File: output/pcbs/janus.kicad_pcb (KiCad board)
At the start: 2 copper layers, 180.2 x 117.5 mm, 55 parts

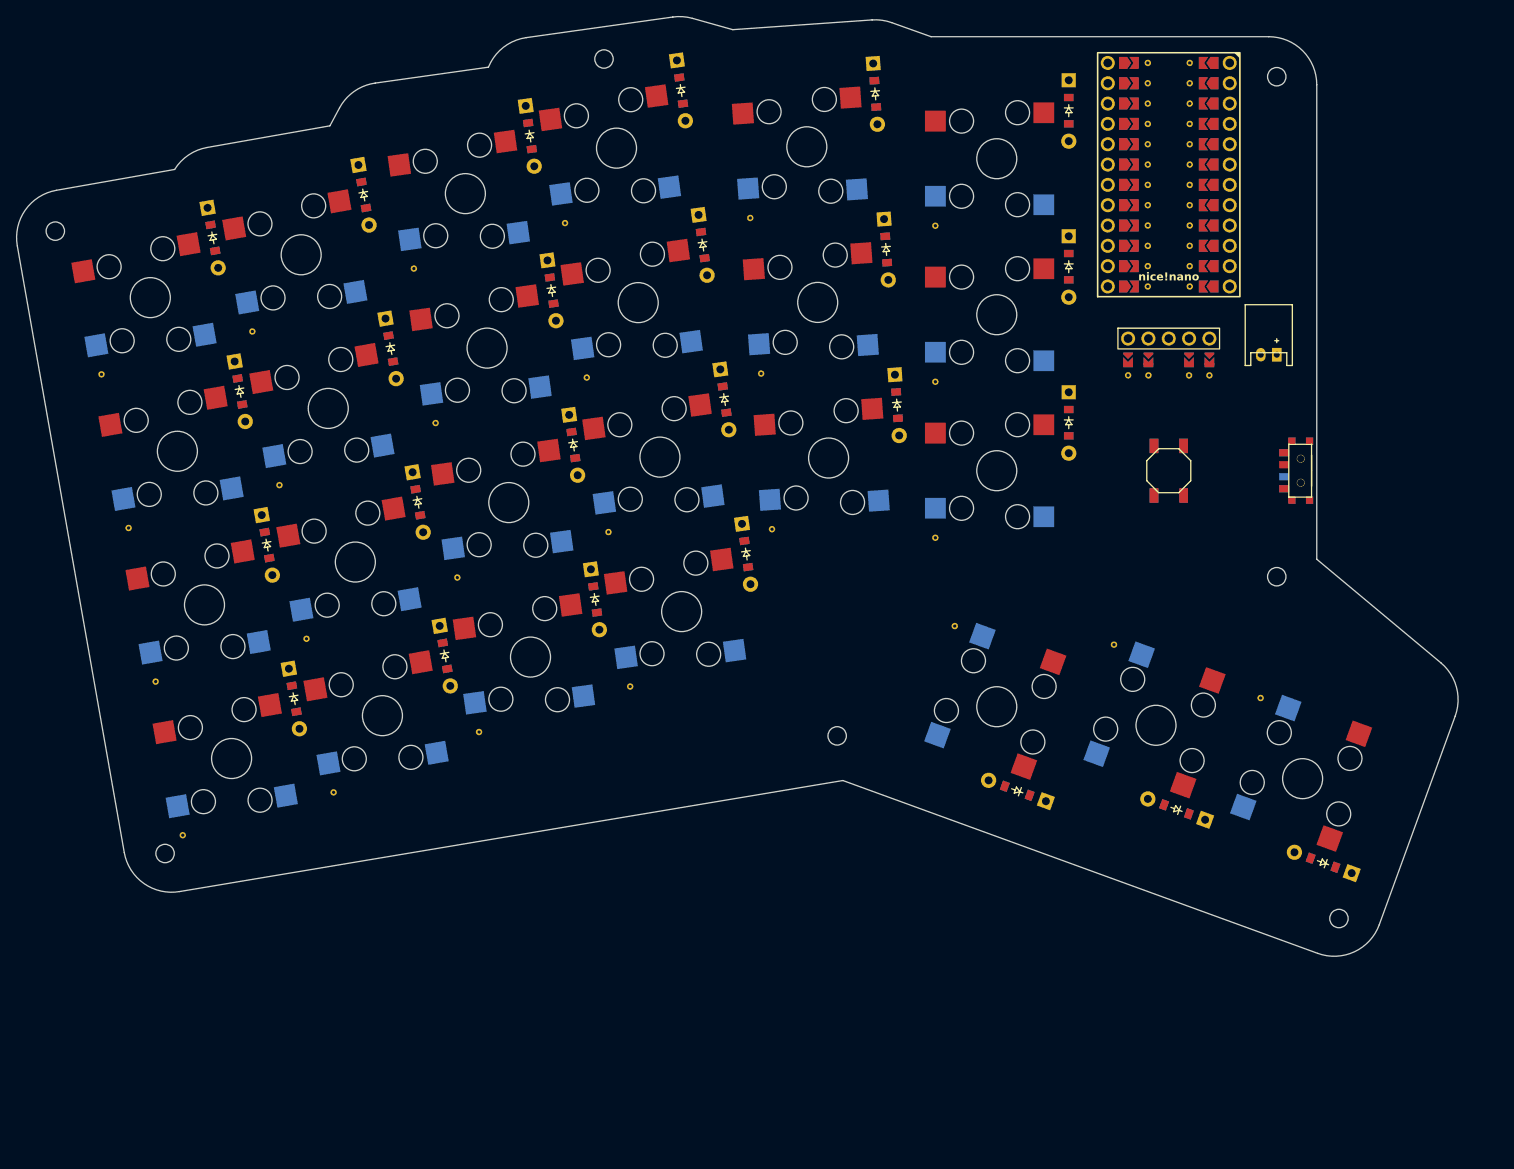
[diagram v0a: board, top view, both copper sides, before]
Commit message: generated output
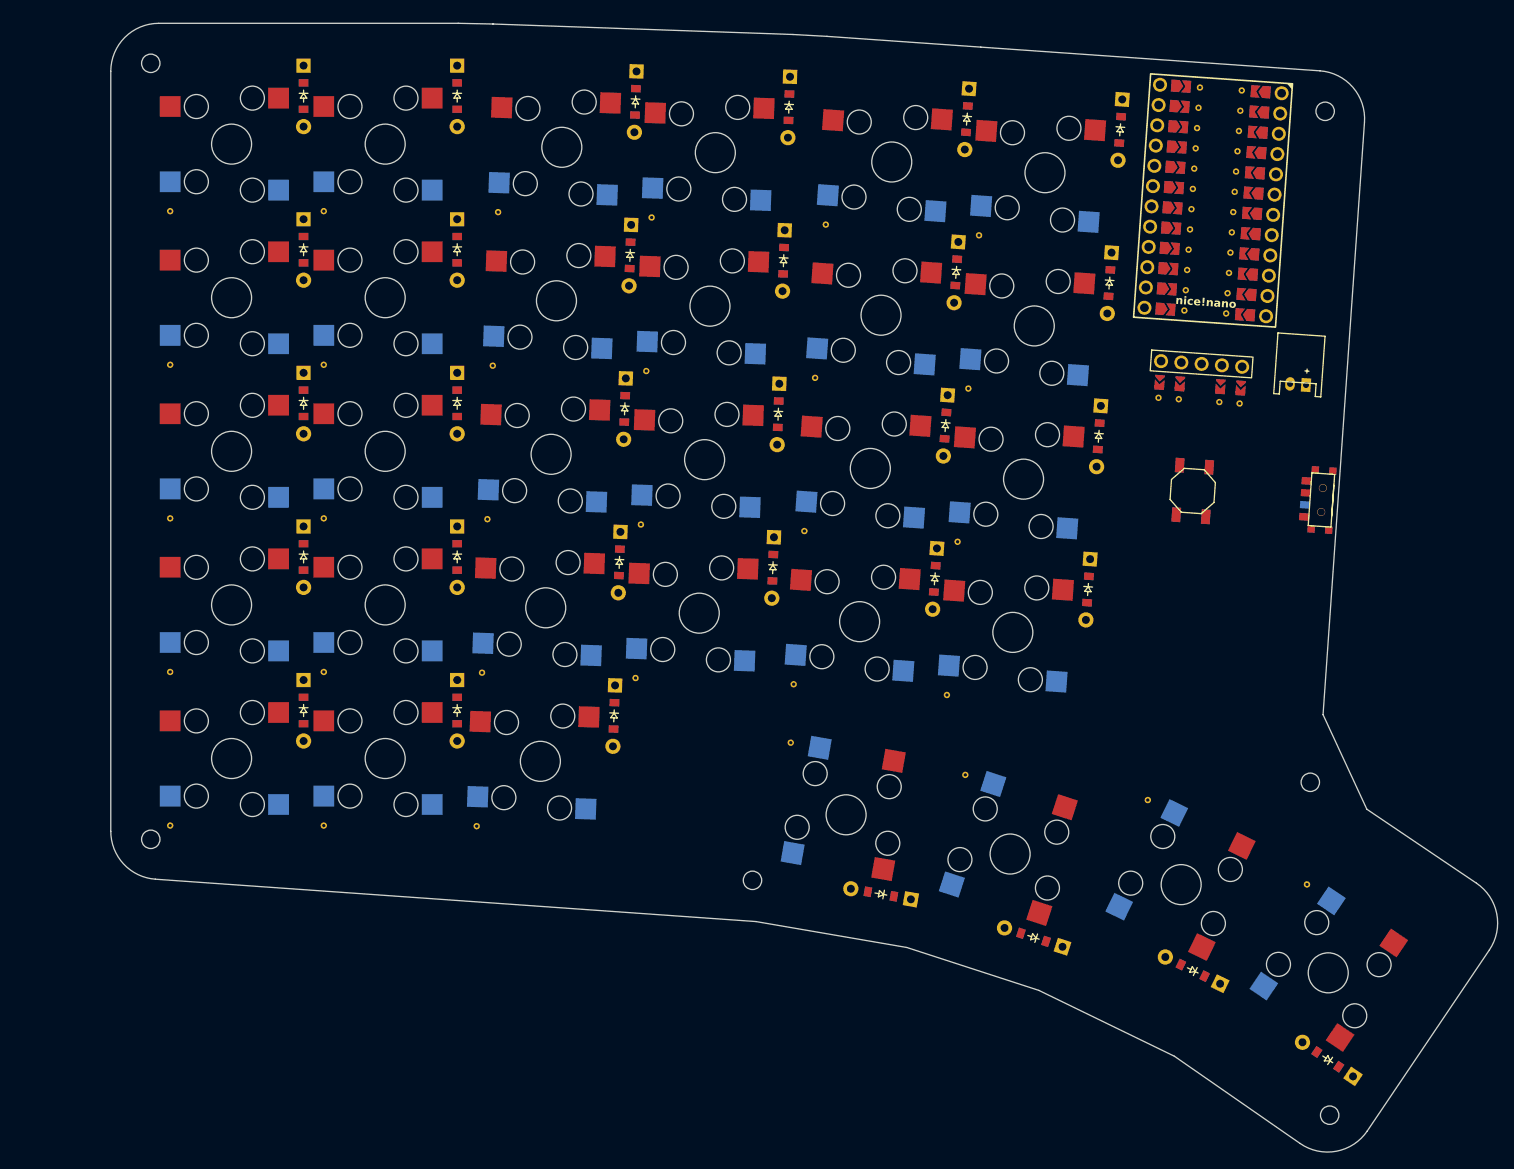
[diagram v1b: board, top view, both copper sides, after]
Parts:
- added D26: , ComboDiode, F.Cu at (159.7, 90.6)
- added D27: , ComboDiode, F.Cu at (161.1, 71.4)
- added D28: , ComboDiode, F.Cu at (131.2, 166.9)
- added D29: , ComboDiode, F.Cu at (150.2, 172.4)
- added D30: , ComboDiode, F.Cu at (170.1, 176.5)
- added D31: , ComboDiode, F.Cu at (187.0, 187.6)
- added S26: ks27, gateron-ks27, F.Cu at (150.3, 95.9)
- added S27: ks27, gateron-ks27, F.Cu at (151.7, 76.8)
- added S28: ks27, gateron-ks27, F.Cu at (126.8, 157.0)
- added S29: ks27, gateron-ks27, F.Cu at (147.3, 161.9)
- added S30: ks27, gateron-ks27, F.Cu at (168.7, 165.8)
- added S31: ks27, gateron-ks27, F.Cu at (187.1, 176.8)
- moved D23 84.2 mm to (141.9, 70.1), turned to -94 degrees
- moved S5 73.9 mm to (50.0, 73.2), turned to 0 degrees
- moved D5 72.2 mm to (59.0, 67.2), turned to -90 degrees
- moved S23 69.3 mm to (132.5, 75.4), turned to -4 degrees
- moved D16 60.7 mm to (117.7, 126.1), turned to -92 degrees
- moved D25 60.2 mm to (158.4, 109.7), turned to -94 degrees
- moved S16 59.0 mm to (108.5, 131.8), turned to -2 degrees
- moved D12 54.4 mm to (98.5, 125.5), turned to -92 degrees
- moved D11 53.7 mm to (97.8, 144.7), turned to -92 degrees
- moved S12 52.7 mm to (89.3, 131.2), turned to -2 degrees
- moved S11 52.1 mm to (88.6, 150.3), turned to -2 degrees
- moved S25 51.2 mm to (149.0, 115.1), turned to -4 degrees
- moved S9 48.5 mm to (69.2, 92.4), turned to 0 degrees
- moved S10 47.4 mm to (69.2, 73.2), turned to 0 degrees
- moved D9 47.0 mm to (78.2, 86.4), turned to -90 degrees
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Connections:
- net inner_cluster renamed index_number
- D1 pad 1: P9 -> (no net)
- D10 pad 1: P8 -> (no net)
- D10 pad 2: ring_bottom -> pinky_number
- D11 pad 1: P7 -> (no net)
- D11 pad 2: ring_home -> ring_mod
- D12 pad 1: P6 -> (no net)
- D12 pad 2: ring_top -> ring_bottom
- D13 pad 1: P9 -> (no net)
- D13 pad 2: middle_mod -> ring_home
- D14 pad 1: P8 -> (no net)
- D14 pad 2: middle_bottom -> ring_top
- D15 pad 1: P7 -> (no net)
- D15 pad 2: middle_home -> ring_number
- D16 pad 1: P6 -> (no net)
- D16 pad 2: middle_top -> middle_bottom
- D17 pad 1: P8 -> (no net)
- D17 pad 2: index_bottom -> middle_home
- D18 pad 1: P7 -> (no net)
- D18 pad 2: index_home -> middle_top
- D19 pad 1: P6 -> (no net)
- D19 pad 2: index_top -> middle_number
- D2 pad 1: P8 -> (no net)
- D20 pad 1: P8 -> (no net)
- D20 pad 2: inner_bottom -> index_bottom
- D21 pad 1: P7 -> (no net)
- D21 pad 2: inner_home -> index_home
- D22 pad 1: P6 -> (no net)
- D22 pad 2: inner_top -> index_top
- D23 pad 1: P9 -> (no net)
- D24 pad 1: P9 -> (no net)
- D24 pad 2: home_cluster -> inner_bottom
- D25 pad 1: P9 -> (no net)
- D25 pad 2: outer_cluster -> inner_home
- D3 pad 1: P7 -> (no net)
- D4 pad 1: P6 -> (no net)
- D5 pad 1: P9 -> (no net)
- D5 pad 2: pinky_mod -> outer_number
- D6 pad 1: P8 -> (no net)
- D6 pad 2: pinky_bottom -> pinky_mod
- D7 pad 1: P7 -> (no net)
- D7 pad 2: pinky_home -> pinky_bottom
- D8 pad 1: P6 -> (no net)
- D8 pad 2: pinky_top -> pinky_home
- D9 pad 1: P9 -> (no net)
- D9 pad 2: ring_mod -> pinky_top
- S1 pad 1: P15 -> (no net)
- S10 pad 1: P16 -> (no net)
- S10 pad 2: ring_bottom -> pinky_number
- S11 pad 1: P16 -> (no net)
- S11 pad 2: ring_home -> ring_mod
- S12 pad 1: P16 -> (no net)
- S12 pad 2: ring_top -> ring_bottom
- S13 pad 1: P10 -> (no net)
- S13 pad 2: middle_mod -> ring_home
- S14 pad 1: P10 -> (no net)
- S14 pad 2: middle_bottom -> ring_top
- S15 pad 1: P10 -> (no net)
- S15 pad 2: middle_home -> ring_number
- S16 pad 1: P10 -> (no net)
- S16 pad 2: middle_top -> middle_bottom
- S17 pad 1: P20 -> (no net)
- S17 pad 2: index_bottom -> middle_home
- S18 pad 1: P20 -> (no net)
- S18 pad 2: index_home -> middle_top
- S19 pad 1: P20 -> (no net)
- S19 pad 2: index_top -> middle_number
- S2 pad 1: P15 -> (no net)
- S20 pad 1: P19 -> (no net)
- S20 pad 2: inner_bottom -> index_bottom
- S21 pad 1: P19 -> (no net)
- S21 pad 2: inner_home -> index_home
- S22 pad 1: P19 -> (no net)
- S22 pad 2: inner_top -> index_top
- S23 pad 1: P20 -> (no net)
- S24 pad 1: P19 -> (no net)
- S24 pad 2: home_cluster -> inner_bottom
- S25 pad 1: P18 -> (no net)
- S25 pad 2: outer_cluster -> inner_home
- S3 pad 1: P15 -> (no net)
- S4 pad 1: P15 -> (no net)
- S5 pad 1: P14 -> (no net)
- S5 pad 2: pinky_mod -> outer_number
- S6 pad 1: P14 -> (no net)
- S6 pad 2: pinky_bottom -> pinky_mod
- S7 pad 1: P14 -> (no net)
- S7 pad 2: pinky_home -> pinky_bottom
- S8 pad 1: P14 -> (no net)
- S8 pad 2: pinky_top -> pinky_home
- S9 pad 1: P16 -> (no net)
- S9 pad 2: ring_mod -> pinky_top
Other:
- board size 180.2 x 117.5 mm -> 173.4 x 141.1 mm
